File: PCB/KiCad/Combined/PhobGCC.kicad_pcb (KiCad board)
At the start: 2 copper layers, 143 x 91.4 mm, 76 parts, among them J1 Conn_01x06_Female, J2 Conn_01x04_Female, J3 Conn_01x01_Male, J4 Conn_01x04_Male, J5 Rumble, Q1 Q_NMOS_GSD, Q2 Q_PMOS_GDS, Q3 Q_NMOS_GSD, SW1 A, SW10 Dup, SW11 Dright, SW12 Ddown, SW2 B, SW3 X, SW4 Y, SW5 Start, SW6 L, SW7 R, SW8 Z, SW9 Dleft, U1 Teensy4.0, U2 2x DRV5053CAQLPGM Hall Effect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, U3 GP2S60-MFG, U4 GP2S60-MFG, U5 Stickbox_Assembly

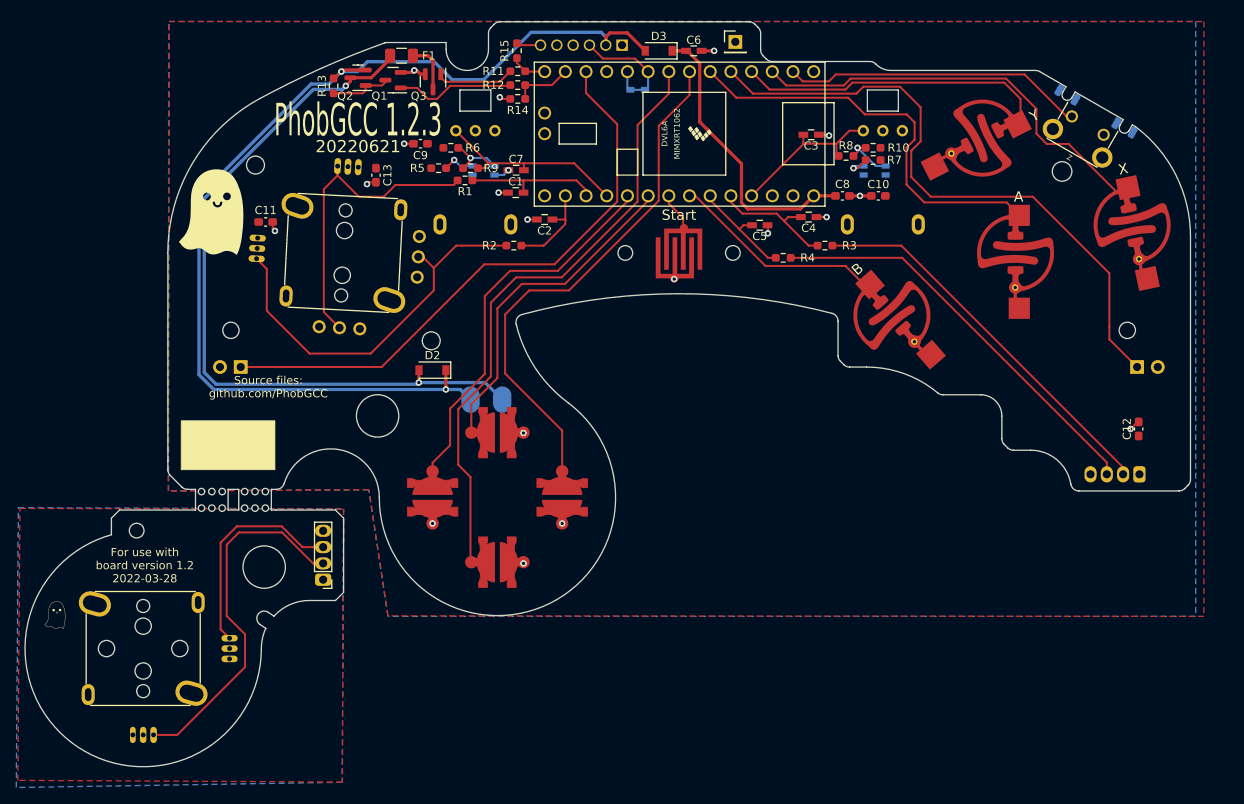
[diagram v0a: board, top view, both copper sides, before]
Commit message: attempt at v1.2.4
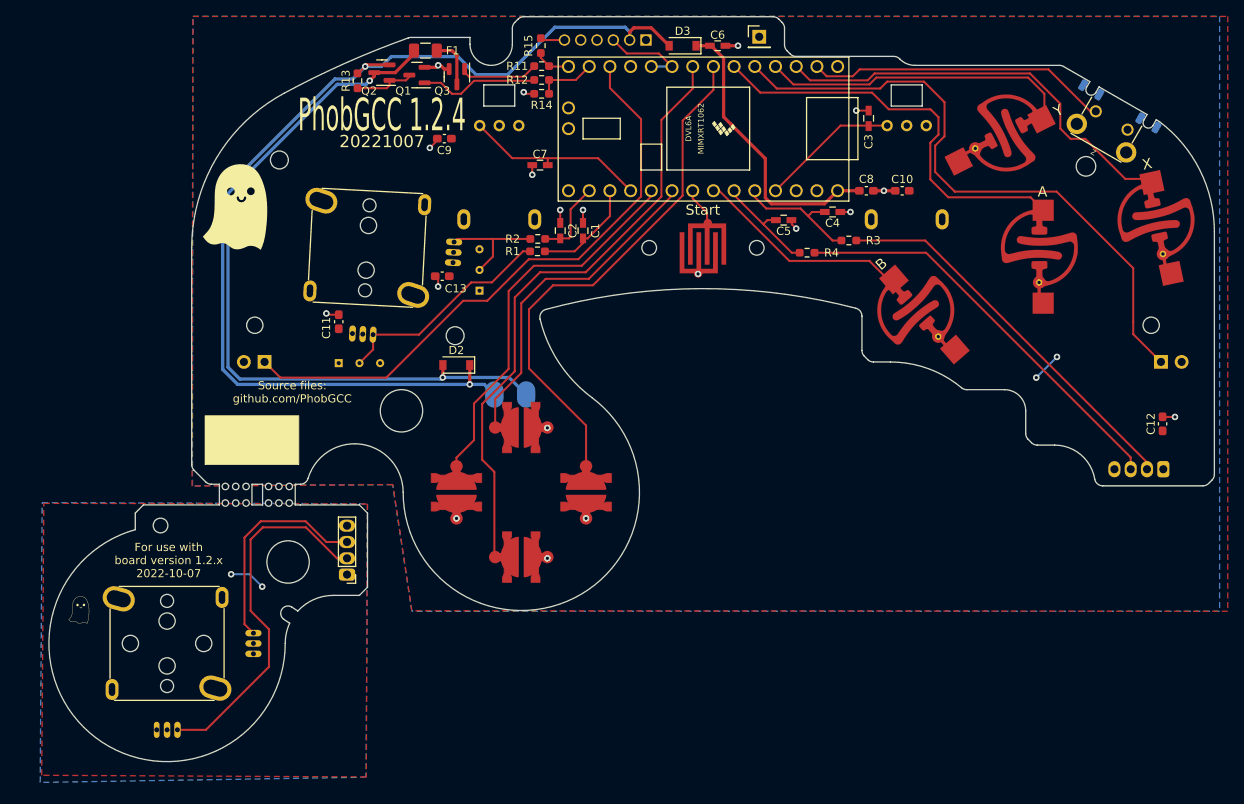
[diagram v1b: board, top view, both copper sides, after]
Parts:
- removed D1: D_Schottky_Shorted, PhobGCC_Footprints:D_SOD-523_Shorted
- removed R10, R5, R6, R7, R8, R9: DNP, PhobGCC_Footprints:R_0603_1608_DNP
- removed U3, U4: GP2S60-MFG, PhobGCC_Footprints:Sharp_Microelectronics-GP2S60-MFG
- added TSTP1: testing pads, Library:testing pads, F.Cu at (70.6, 66.3)
- added TSTP2: testing pads, Library:testing pads, F.Cu at (85.3, 54.9)
- moved C11 15.2 mm to (68.1, 61.2), turned to 90 degrees
- moved C13 14.8 mm to (80.8, 55.7), turned to 180 degrees
- moved R1 12.4 mm to (92.4, 52.6)
- moved C1 9.48 mm to (98.0, 50.1), turned to 90 degrees
- moved C3 7.34 mm to (133.1, 36.3), turned to 90 degrees
- moved R2 3.04 mm to (92.5, 51.1)
- moved H4 3.00 mm to (167.8, 61.7)
- moved H7 3.00 mm to (159.8, 42.2)
- moved J2 3.00 mm to (169.2, 79.3)
- moved RV2 3.00 mm to (137.8, 37.2)
- moved SW1 3.00 mm to (154.0, 52.1)
- moved SW4 3.00 mm to (150.0, 38.0)
- moved SW8 3.00 mm to (162.9, 36.6)
- moved G*** 3.00 mm to (36.2, 96.7)
- moved H1 3.00 mm to (75.8, 72.2)
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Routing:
- net /Stick_y: track 47.6 -> 14.3 mm
- net /Stick_x: track 38.1 -> 27.7 mm
- net Net-(R6-Pad2): track 6.75 -> 0.00 mm, vias 1 -> 0
- net Net-(R10-Pad2): track 6.58 -> 0.00 mm, vias 1 -> 0
- net VCC: track 0.00 -> 4.44 mm, vias 0 -> 2
- net Net-(R5-Pad2): track 3.96 -> 0.00 mm, vias 1 -> 0
- net /Data: track 15.0 -> 11.1 mm
- net +3V3: track 0.00 -> 3.59 mm, vias 0 -> 2
- net Net-(R7-Pad2): track 3.28 -> 0.00 mm, vias 1 -> 0
- net /Stick_x_filt: track 16.7 -> 14.0 mm
- net /Ranalog: track 19.4 -> 17.0 mm
- net GND: track 24.0 -> 26.0 mm
- net /Stick_y_filt: track 11.7 -> 9.83 mm
- net /L: track 72.1 -> 73.7 mm
- net /Lanalog: track 24.2 -> 22.7 mm
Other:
- board text added: "20221007"
- board text added: "For use with board version 1.2.x 2022-10-07"
- board text added: "PhobGCC 1.2.4"
- board text removed: "20220621"
- board text removed: "For use with board version 1.2 2022-03-28"
- board text removed: "PhobGCC 1.2.3"
